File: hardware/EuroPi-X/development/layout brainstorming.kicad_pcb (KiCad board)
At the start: 2 copper layers, 40.6 x 110 mm, 32 parts

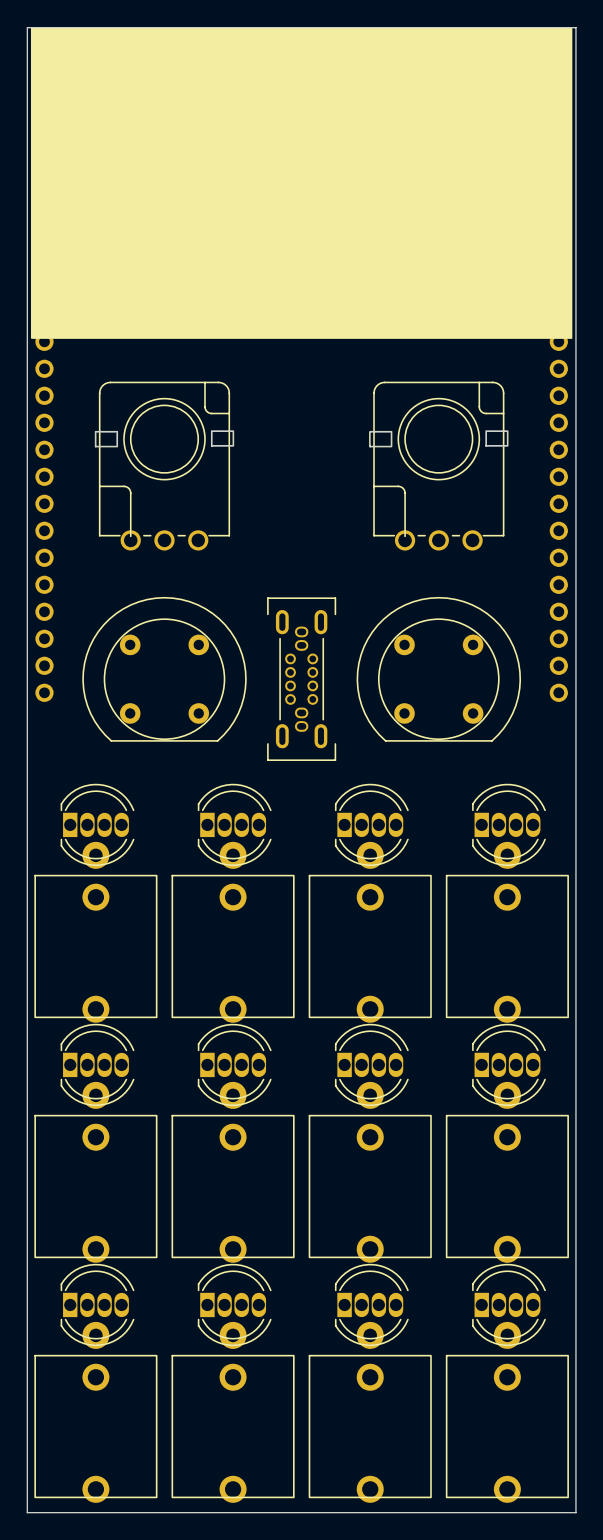
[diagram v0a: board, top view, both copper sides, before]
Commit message: save
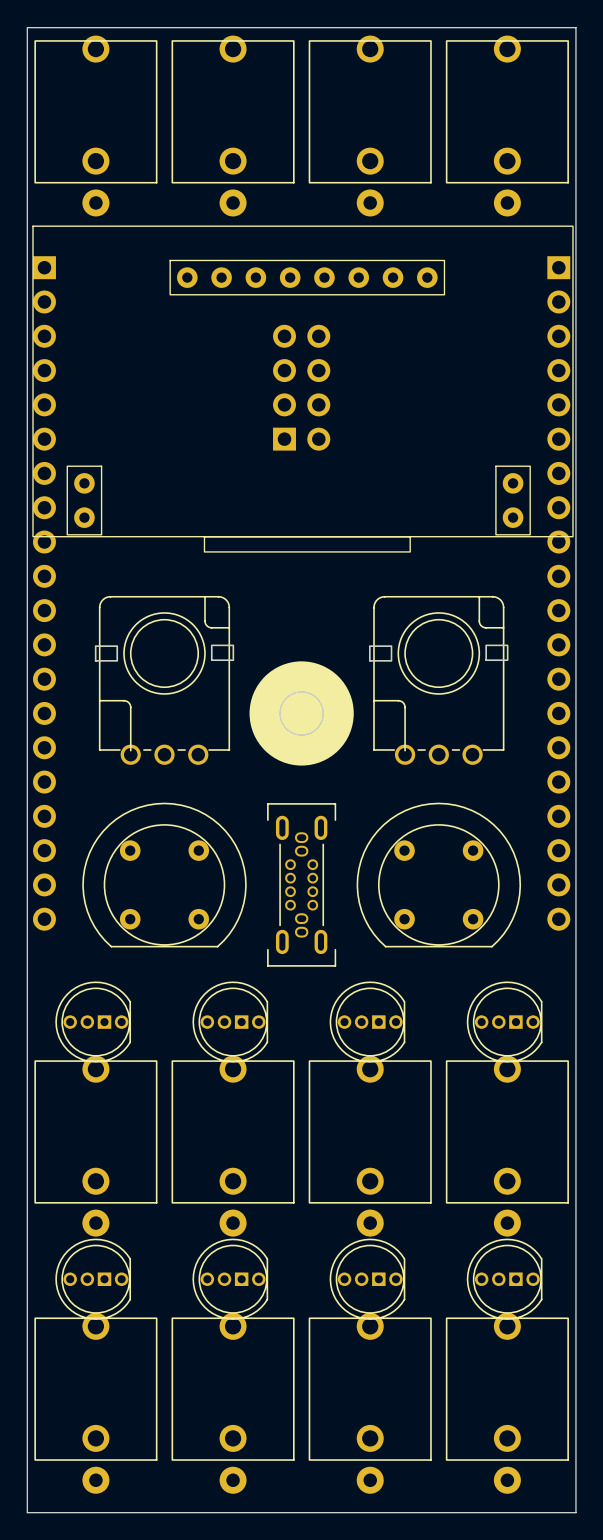
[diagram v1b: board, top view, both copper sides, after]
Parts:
- removed the REF** at (13.3, 94.6)
- removed the REF** at (23.5, 94.6)
- removed the REF** at (13.3, 76.8)
- removed the REF** at (23.5, 59.1)
- removed the REF** at (3.18, 94.6)
- removed the REF** at (39.4, 1.27)
- removed the REF** at (1.27, 1.27)
- removed the REF** at (5.08, 1.27)
- removed the REF** at (33.7, 76.8)
- removed the REF** at (3.18, 59.1)
- removed the REF** at (13.3, 59.1)
- removed the REF** at (33.7, 59.1)
- removed the REF** at (23.5, 76.8)
- removed the REF** at (33.7, 94.6)
- removed the REF** at (3.18, 76.8)
- added REF**: 254-5726 RGB Led 5mm, allen-synthesis:254-5726 RGB Led 5mm, F.Cu at (15.2, 92.7)
- added REF**: 254-5726 RGB Led 5mm, allen-synthesis:254-5726 RGB Led 5mm, F.Cu at (15.2, 73.7)
- added REF**: PinHeader_2x04_P2.54mm_Vertical, Connector_PinHeader_2.54mm:PinHeader_2x04_P2.54mm_Vertical, B.Cu at (19.1, 30.5)
- added REF**: PinHeader_1x20_P2.54mm_Vertical, Connector_PinHeader_2.54mm:PinHeader_1x20_P2.54mm_Vertical, B.Cu at (1.27, 17.8)
- added REF**: PinHeader_1x20_P2.54mm_Vertical, Connector_PinHeader_2.54mm:PinHeader_1x20_P2.54mm_Vertical, B.Cu at (39.4, 17.8)
- added REF**: 254-5726 RGB Led 5mm, allen-synthesis:254-5726 RGB Led 5mm, F.Cu at (5.08, 92.7)
- added REF**: 254-5726 RGB Led 5mm, allen-synthesis:254-5726 RGB Led 5mm, F.Cu at (25.4, 92.7)
- added REF**: 254-5726 RGB Led 5mm, allen-synthesis:254-5726 RGB Led 5mm, F.Cu at (35.6, 73.7)
- added REF**: 254-5726 RGB Led 5mm, allen-synthesis:254-5726 RGB Led 5mm, F.Cu at (25.4, 73.7)
- added REF**: 254-5726 RGB Led 5mm, allen-synthesis:254-5726 RGB Led 5mm, F.Cu at (35.6, 92.7)
- added REF**: Toadstool Tech Enoki, allen-synthesis:Toadstool Tech Enoki, F.Cu at (0.42, 14.7)
- added REF**: 254-5726 RGB Led 5mm, allen-synthesis:254-5726 RGB Led 5mm, F.Cu at (5.08, 73.7)
- moved THONK 60.3 mm to (5.08, 6.99), turned to 90 degrees
- moved THONK 60.3 mm to (25.4, 6.99), turned to 90 degrees
- moved THONK 60.3 mm to (15.2, 6.99), turned to 90 degrees
- moved THONK 60.3 mm to (35.6, 6.99), turned to 90 degrees
- moved POT 15.9 mm to (30.5, 46.4)
- moved POT 15.9 mm to (10.2, 46.4)
- moved REF** 15.2 mm to (20.3, 63.5)
- moved SW 15.2 mm to (10.2, 63.5)
- moved SW 15.2 mm to (30.5, 63.5)
- moved THONK 2.54 mm to (35.6, 82.5), turned to 90 degrees
- moved THONK 2.54 mm to (15.2, 82.5), turned to 90 degrees
- moved THONK 2.54 mm to (25.4, 82.5), turned to 90 degrees
- moved THONK 2.54 mm to (5.08, 82.5), turned to 90 degrees
- moved THONK 1.27 mm to (5.08, 101.6), turned to 90 degrees
- moved THONK 1.27 mm to (25.4, 101.6), turned to 90 degrees
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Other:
- outline, holes or cut-outs redrawn
- board text added: "25 + 24 leds"
- board text added: "49 pins"
- board text removed: "11"
- board text removed: "12x LED"
- board text removed: "3V3 GND SDA SCL"
- board text removed: "48"
- board text removed: "4X OUT"
- board text removed: "4x IN"
- board text removed: "59"
- board text removed: "B1 B2"
- board text removed: "D+ D- 5V"
- board text removed: "K1 K2"

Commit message: save
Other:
- board text removed: "25 + 24 leds"
- board text removed: "49 pins"
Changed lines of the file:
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@@
   (gr_circle (center 20.32 50.8) (end 21.92 50.8)
     (stroke (width 0.05) (type default)) (fill none) (layer "Edge.Cuts"))
-  (gr_text "49 pins" (at 50.8 17.78) (layer "User.1")
-    (effects (font (size 1.5 1.5) (thickness 0.3) bold) (justify left bottom))
-  )
-  (gr_text "25 + 24 leds" (at 50.8 13.97) (layer "User.1")
-    (effects (font (size 1.5 1.5) (thickness 0.3) bold) (justify left bottom))
-  )
 )
